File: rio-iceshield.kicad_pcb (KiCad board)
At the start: 4 copper layers, 87.6 x 56 mm, 105 parts, among them J2 Conn_01x06, J3 Conn_01x06, J4 Conn_01x06, J5 Conn_01x06, J6 Conn_01x06, U1 ICE40UP5K-SG48ITR, U10 PC817, U11 PC817, U12 PC817, U13 PC817, U14 PC817, U2 AT25SF041B-SHD 4 Mb, U3 LD3985M122R_SOT23, U4 ULN2803A, U5 ULN2803A, U7 PC817, U8 PC817, U9 PC817, X2 XO91, j1 GPIO

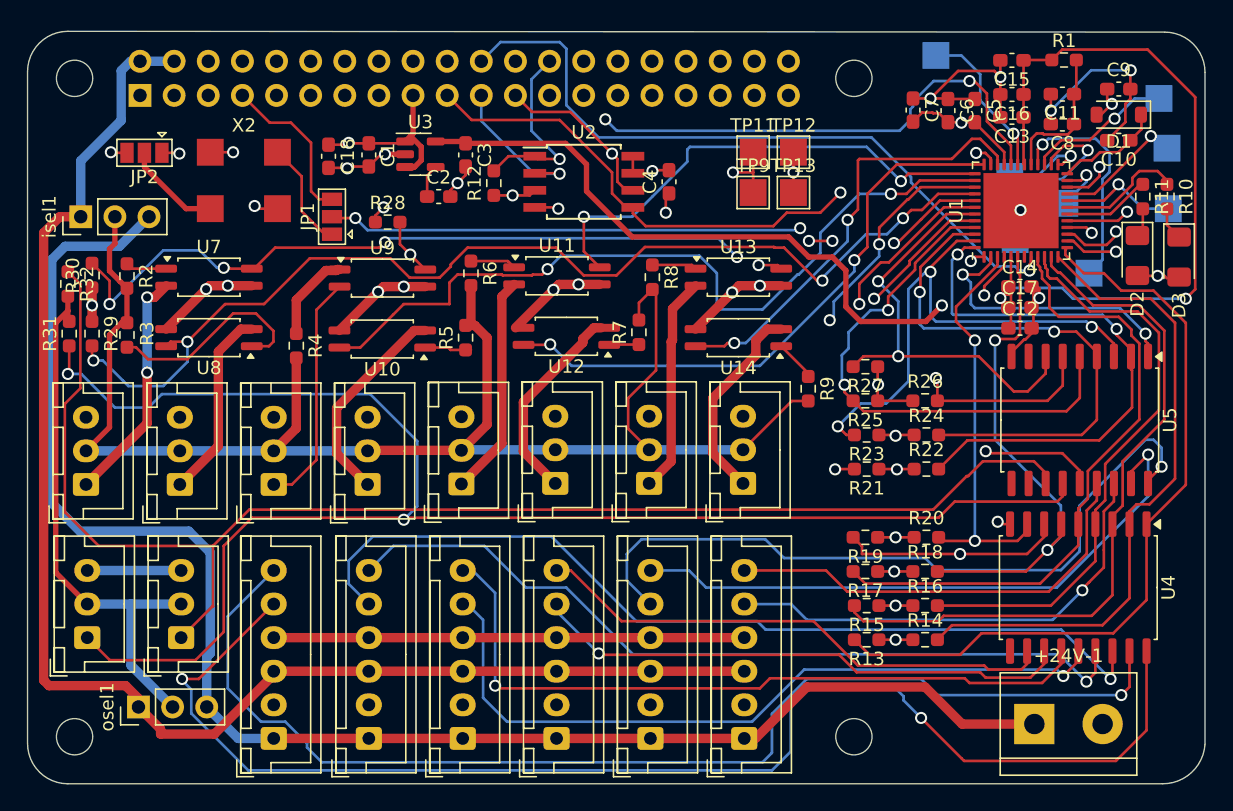
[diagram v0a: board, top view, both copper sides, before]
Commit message: wip
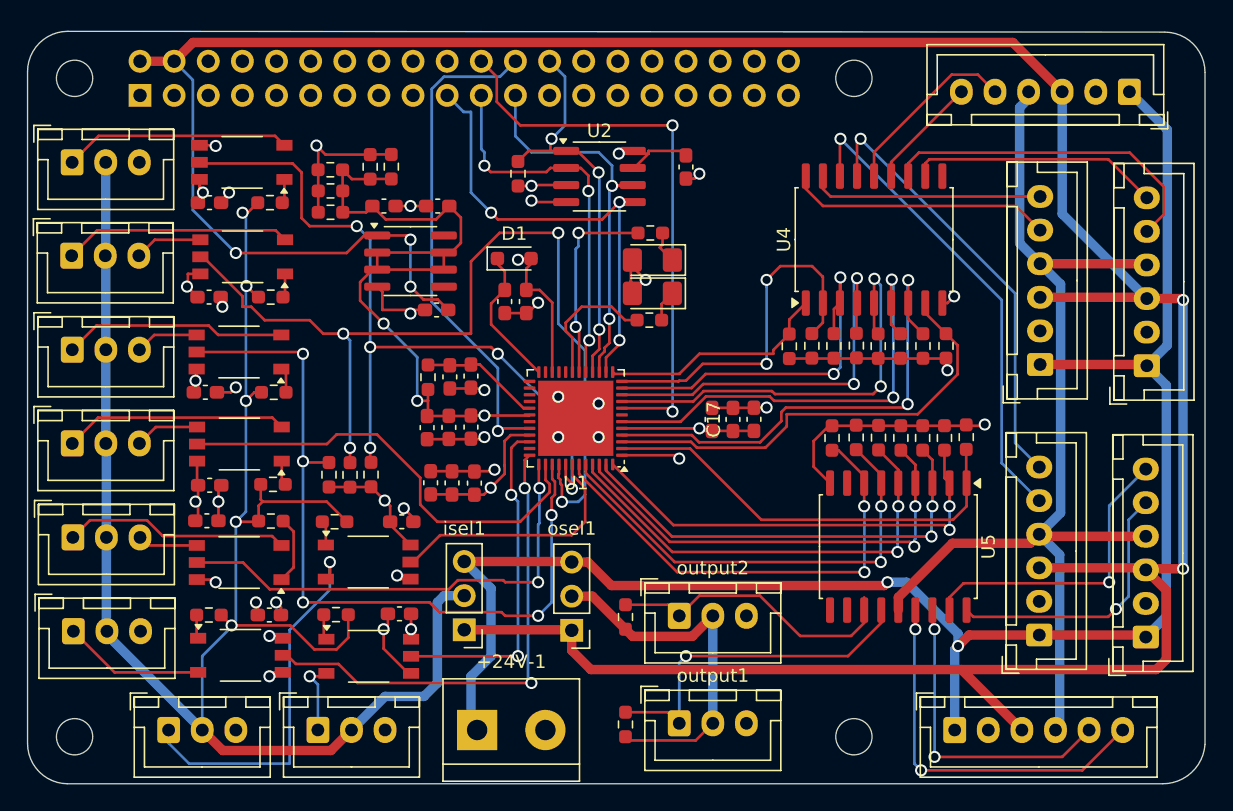
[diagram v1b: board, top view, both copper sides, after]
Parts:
- removed JP1, JP2: SolderJumper_3_Open, Jumper:SolderJumper-3_P1.3mm_Open_Pad1.0x1.5mm
- removed TP10, TP11, TP12, TP13, TP2, TP3, TP4, TP5, TP6, TP7, TP8, TP9: TestPoint_Small, TestPoint:TestPoint_Pad_2.0x2.0mm
- removed U10, U11, U12, U13, U14, U8, U9: PC817, Package_SO:SOP-4_4.4x2.6mm_P1.27mm
- removed U3: LD3985M122R_SOT23, Package_TO_SOT_SMD:SOT-23-5
- removed X2: XO91, Oscillator:Oscillator_SMD_EuroQuartz_XO91-4Pin_7.0x5.0mm
- added C19: 100n, Capacitor_SMD:C_0603_1608Metric_Pad1.08x0.95mm_HandSolder, F.Cu at (113.5, 63.8)
- added C20: 100n, Capacitor_SMD:C_0603_1608Metric_Pad1.08x0.95mm_HandSolder, F.Cu at (113.2, 70.9)
- added C21: 100n, Capacitor_SMD:C_0603_1608Metric_Pad1.08x0.95mm_HandSolder, F.Cu at (113.6, 77.8)
- added C22: 100n, Capacitor_SMD:C_0603_1608Metric_Pad1.08x0.95mm_HandSolder, F.Cu at (113.3, 80.4)
- added C23: 100n, Capacitor_SMD:C_0603_1608Metric_Pad1.08x0.95mm_HandSolder, F.Cu at (118.0, 87.4)
- added C24: 100n, Capacitor_SMD:C_0603_1608Metric_Pad1.08x0.95mm_HandSolder, F.Cu at (127.8, 80.5)
- added C25: 100n, Capacitor_SMD:C_0603_1608Metric_Pad1.08x0.95mm_HandSolder, F.Cu at (127.7, 87.4)
- added R33: 1k2, Resistor_SMD:R_0603_1608Metric_Pad0.98x0.95mm_HandSolder, F.Cu at (122.5, 57.5)
- added R34: 1k2, Resistor_SMD:R_0603_1608Metric_Pad0.98x0.95mm_HandSolder, F.Cu at (127.1, 54.1)
- added R35: 1k2, Resistor_SMD:R_0603_1608Metric_Pad0.98x0.95mm_HandSolder, F.Cu at (125.5, 54.1)
- added R36: 1k2, Resistor_SMD:R_0603_1608Metric_Pad0.98x0.95mm_HandSolder, F.Cu at (122.5, 54.3)
- added R37: 1k2, Resistor_SMD:R_0603_1608Metric_Pad0.98x0.95mm_HandSolder, F.Cu at (122.5, 55.9)
- added U15: ELM453-TA-V, Package_SO:MFSOP6-5_4.4x3.6mm_P1.27mm, F.Cu at (116.0, 60.8)
- added U16: ELM453-TA-V, Package_SO:MFSOP6-5_4.4x3.6mm_P1.27mm, F.Cu at (115.7, 67.9)
- added U17: ELM453-TA-V, Package_SO:MFSOP6-5_4.4x3.6mm_P1.27mm, F.Cu at (115.8, 74.7)
- added U18: ELM453-TA-V, Package_SO:MFSOP6-5_4.4x3.6mm_P1.27mm, F.Cu at (115.7, 83.5)
- added U19: ELM453-TA-V, Package_SO:MFSOP6-5_4.4x3.6mm_P1.27mm, F.Cu at (115.8, 90.4)
- added U20: ELM453-TA-V, Package_SO:MFSOP6-5_4.4x3.6mm_P1.27mm, F.Cu at (125.3, 83.5)
- added U21: ELM453-TA-V, Package_SO:MFSOP6-5_4.4x3.6mm_P1.27mm, F.Cu at (125.4, 90.5)
- added U6: ELM453-TA-V, Package_SO:MFSOP6-5_4.4x3.6mm_P1.27mm, F.Cu at (116.0, 53.8)
- D1: footprint Diode_SMD:D_SOD-123 -> Diode_SMD:D_SOD-323_HandSoldering
- U2: footprint Package_SO:SOIC-8W_5.3x5.3mm_P1.27mm -> Package_SO:SOIC-8_3.9x4.9mm_P1.27mm
- U7: value PC817 -> LM317LD13TR; footprint Package_SO:SOP-4_4.4x2.6mm_P1.27mm -> Package_SO:SOIC-8_3.9x4.9mm_P1.27mm
- moved J3 69.1 mm to (182.0, 48.5), turned to 180 degrees
- moved Jo1 63.5 mm to (175.4, 68.8)
- moved R1 52.9 mm to (129.8, 69.7), turned to 90 degrees
- moved J4 52.0 mm to (183.3, 68.9)
- moved R31 50.6 mm to (144.5, 95.6), turned to -90 degrees
- moved J2 50.5 mm to (175.3, 88.9)
- moved C11 50.2 mm to (131.4, 69.7), turned to -90 degrees
- moved C16 50.1 mm to (129.7, 73.5), turned to -90 degrees
- moved C15 48.6 mm to (133.0, 73.5), turned to -90 degrees
- moved R32 48.3 mm to (144.5, 87.6)
- moved C8 47.8 mm to (133.0, 69.7), turned to -90 degrees
- moved C13 47.8 mm to (131.4, 73.5), turned to -90 degrees
- moved C10 47.2 mm to (135.5, 64.1), turned to -90 degrees
- moved C9 46.8 mm to (137.1, 64.1), turned to -90 degrees
- moved C5 46.4 mm to (133.3, 77.6)
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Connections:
- C1 pad 1: 3v3 -> 5v
- C2 pad 1: Net-(U3-BYP) -> 1v2
- U7 pad 1: Net-(R2-Pad1) -> 5v
- U7 pad 2: Net-(input1-Pin_1) -> 1v2
- U7 pad 3: gnd -> 1v2
- U7 pad 4: 41 -> gnd
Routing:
- net 5v: track 109.4 -> 235.5 mm, vias 0 -> 5
- net out1: track 120.3 -> 26.1 mm, vias 2 -> 1
- net out2: track 104.4 -> 22.3 mm
- net j1_step: track 98.6 -> 19.7 mm, vias 2 -> 0
- net j1_dir: track 87.4 -> 17.4 mm, vias 1 -> 0
- net 35: track 52.6 -> 0.00 mm, vias 3 -> 0
- net SPI_CS1: track 76.6 -> 29.7 mm, vias 2 -> 3
- net j3_dir: track 54.2 -> 8.44 mm, vias 1 -> 0
- net j3_step: track 55.8 -> 13.7 mm, vias 1 -> 0
- net 13: track 57.4 -> 17.4 mm
- net j5_step: track 55.0 -> 20.4 mm
- net SPI_SCK: track 61.4 -> 27.5 mm
- net SPI_MISO: track 61.2 -> 28.4 mm, vias 4 -> 3
- net j2_step: track 67.8 -> 35.8 mm
- net in_power: track 112.2 -> 141.8 mm, vias 0 -> 5
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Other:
- board text added: "rio-iceshield-v2 https://github.com/digiexchris/rio-iceshield-v2 based on rio-iceshield https://github.com/multigcs/rio-iceshield"
